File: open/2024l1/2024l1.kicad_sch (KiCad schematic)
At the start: 129 parts, among them IC1 LM2587S-ADJ, J1 Conn_01x04, J2 Conn_01x04, J3 Conn_01x02, SW1 STM RST, U1 CD74HC4067SM, U2 CD74HC4067SM, U3 STM32F103CBTx, U4 PC817, Y1 8Mhz

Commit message: L1-Changed Boost Inductor, Shifted L2 Connector
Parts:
- L1: footprint 2024l1:0630 One Piece Inductor -> 2024l1:1040 One Piece Inductor
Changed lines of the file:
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@@
       (effects (font (size 1.27 1.27)))
     )
-    (property "Footprint" "2024l1:0630 One Piece Inductor" (at 205.74 152.4 0)
+    (property "Footprint" "2024l1:1040 One Piece Inductor" (at 205.74 152.4 0)
       (effects (font (size 1.27 1.27)) hide)
     )

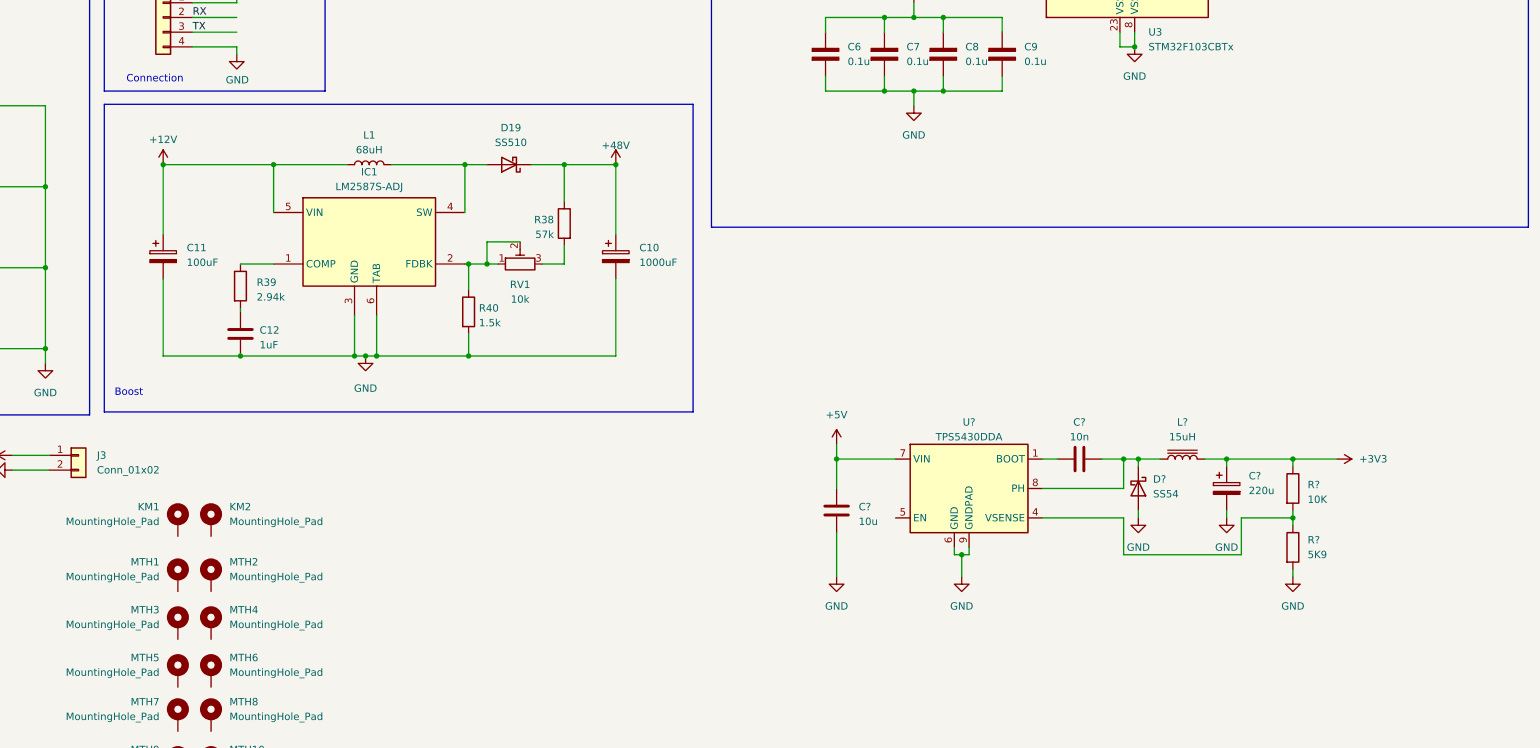
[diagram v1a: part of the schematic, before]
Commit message: open - l1 - ceramic caps
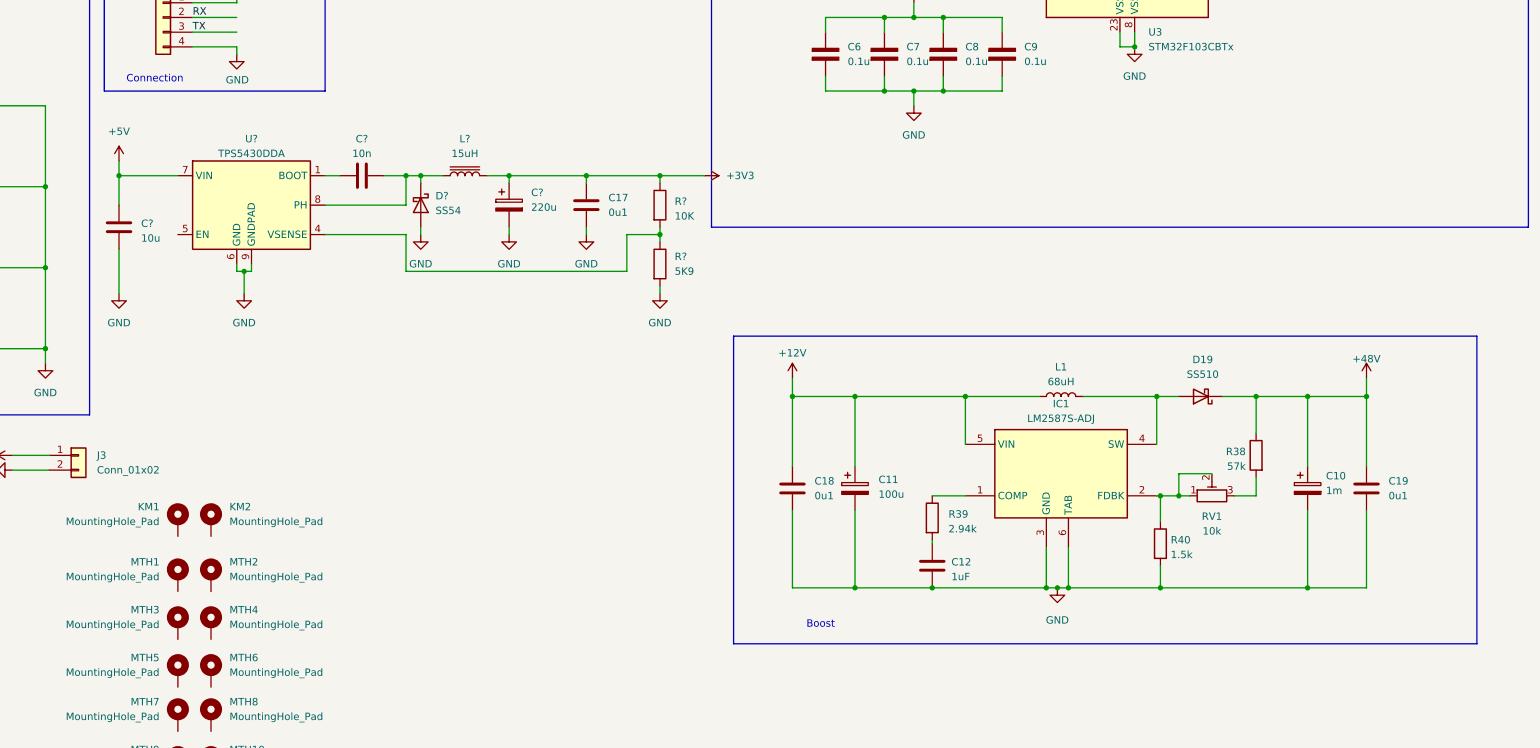
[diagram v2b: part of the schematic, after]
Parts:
- added C17, C18, C19: 0u1, 2024l1:cap0603, symbol Device:C
- C10: value 1000uF -> 1m
- C11: value 100uF -> 100u
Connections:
- net +12V: now also C18.1
- net +3V3: now also C17.1
- net +48V: now also C19.1
- net GND: now also C17.2, C18.2, C19.2
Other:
- moved on the sheet: C10, C11, C12, C?, D19, D?, IC1, L1, L?, R38, R39, R40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

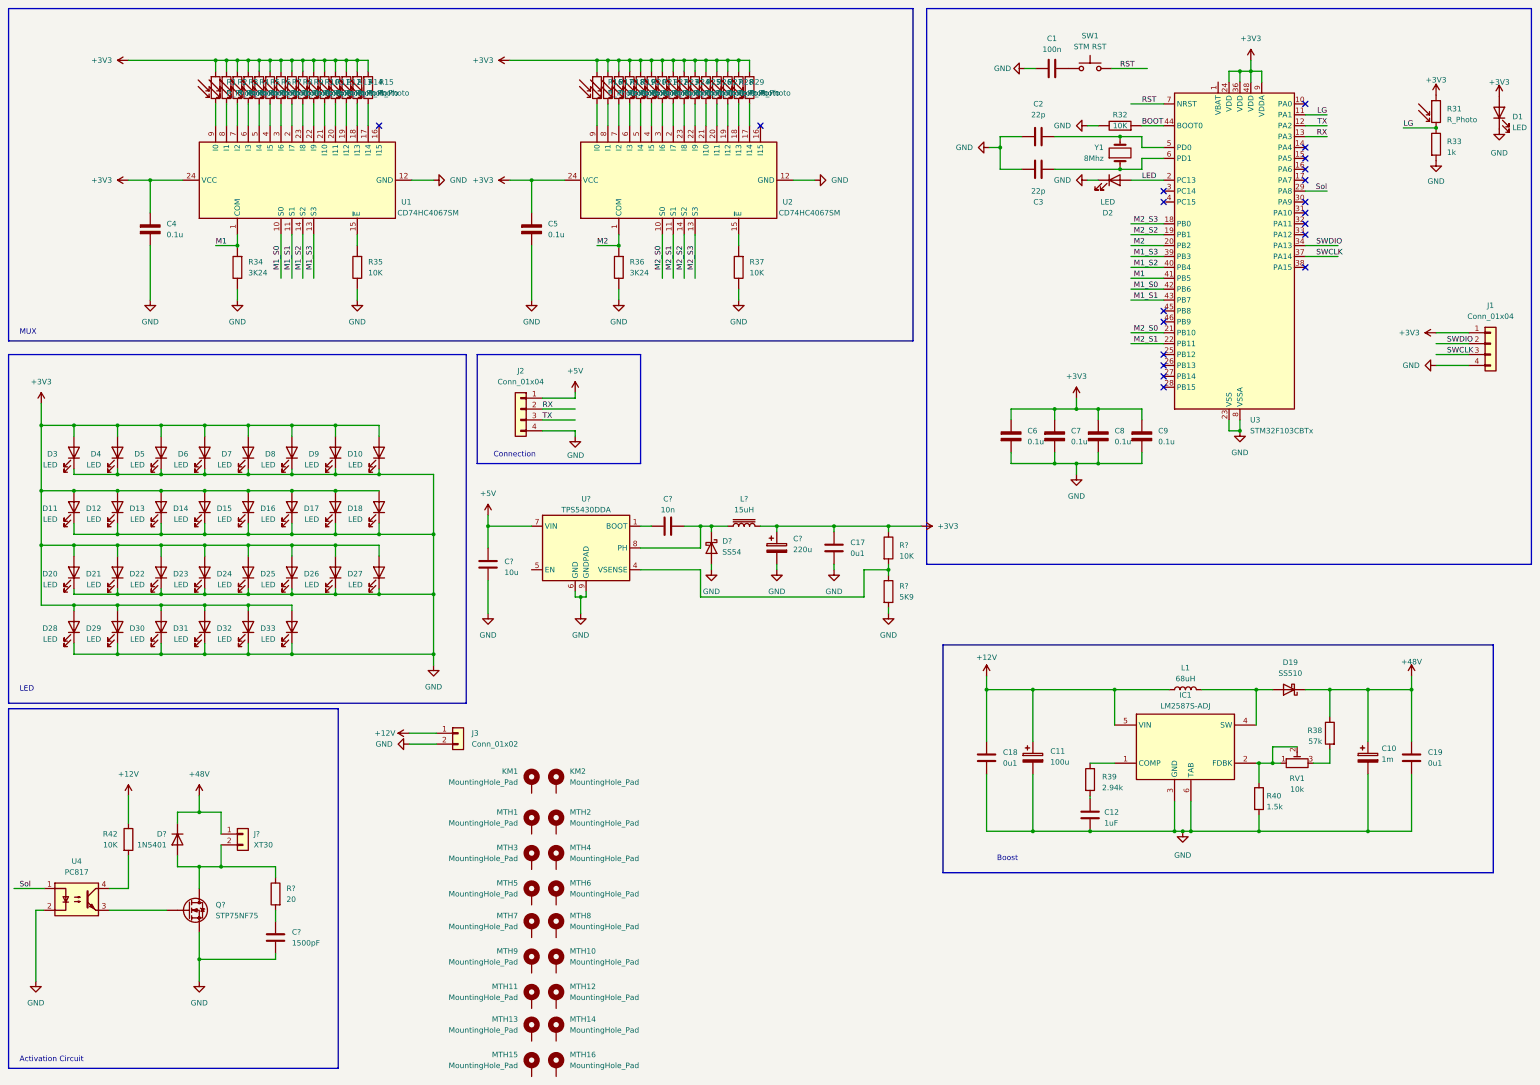
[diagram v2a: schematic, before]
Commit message: open - l1 - silkscreen UI
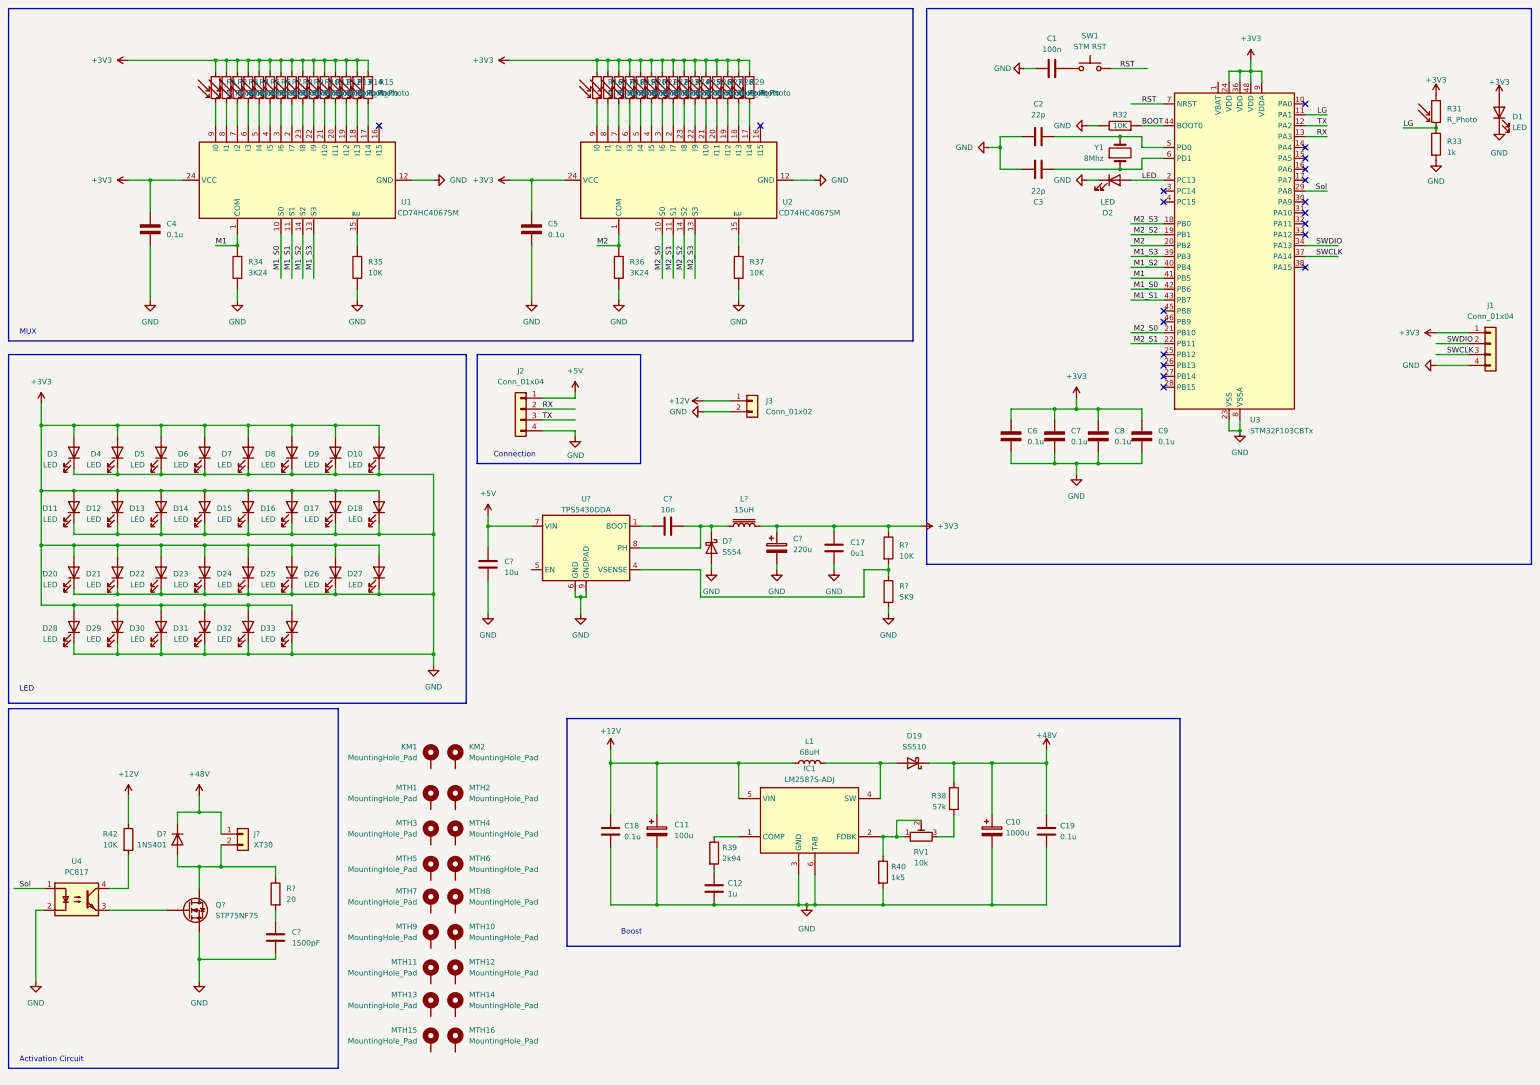
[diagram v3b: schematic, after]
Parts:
- C10: value 1m -> 1000u
- C11: footprint Capacitor_SMD:CP_Elec_6.3x7.7 -> Capacitor_SMD:CP_Elec_10x10.5
- C12: value 1uF -> 1u
- C18, C19: value 0u1 -> 0.1u
- R39: value 2.94k -> 2k94
- R40: value 1.5k -> 1k5
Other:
- moved on the sheet: C10, C11, C12, C18, C19, D19, IC1, J3, KM1, KM2, L1, MTH1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
